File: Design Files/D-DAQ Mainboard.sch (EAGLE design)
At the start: 119 parts, among them Y1 XTC7009, Y2 DS1099

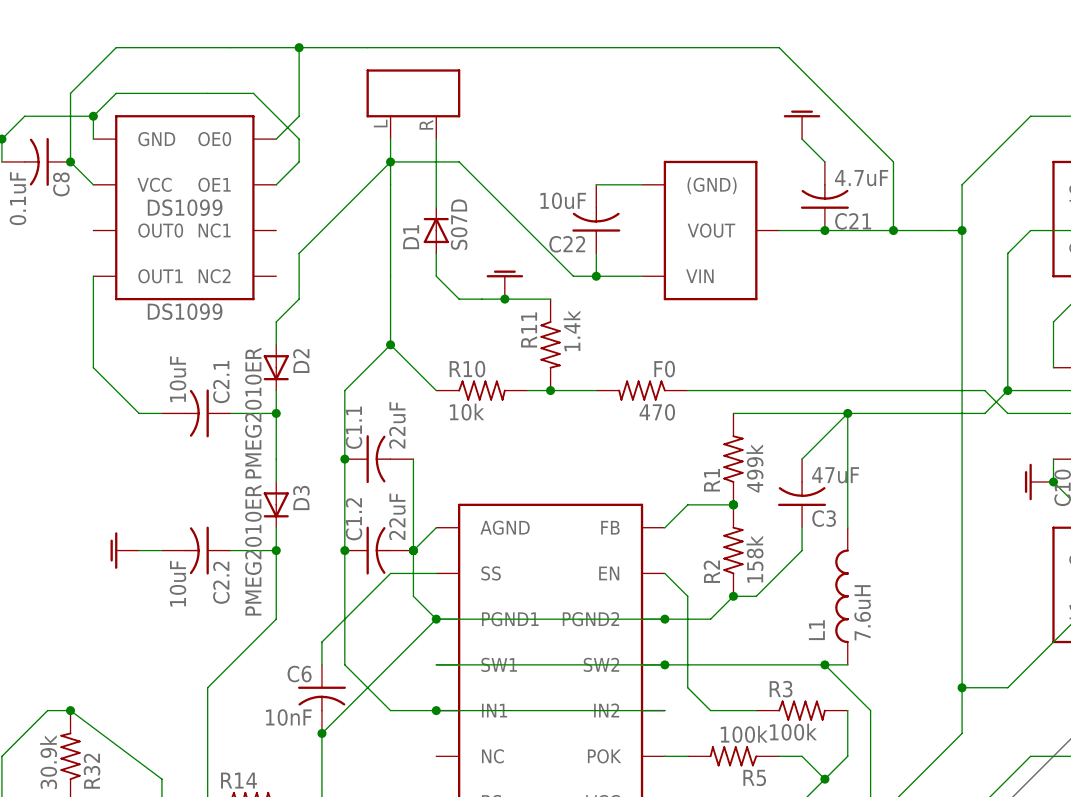
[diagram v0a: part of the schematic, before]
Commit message: v3.6.5 - Package & placement tweaks to design files and then permissions changes due to new system local copies reside
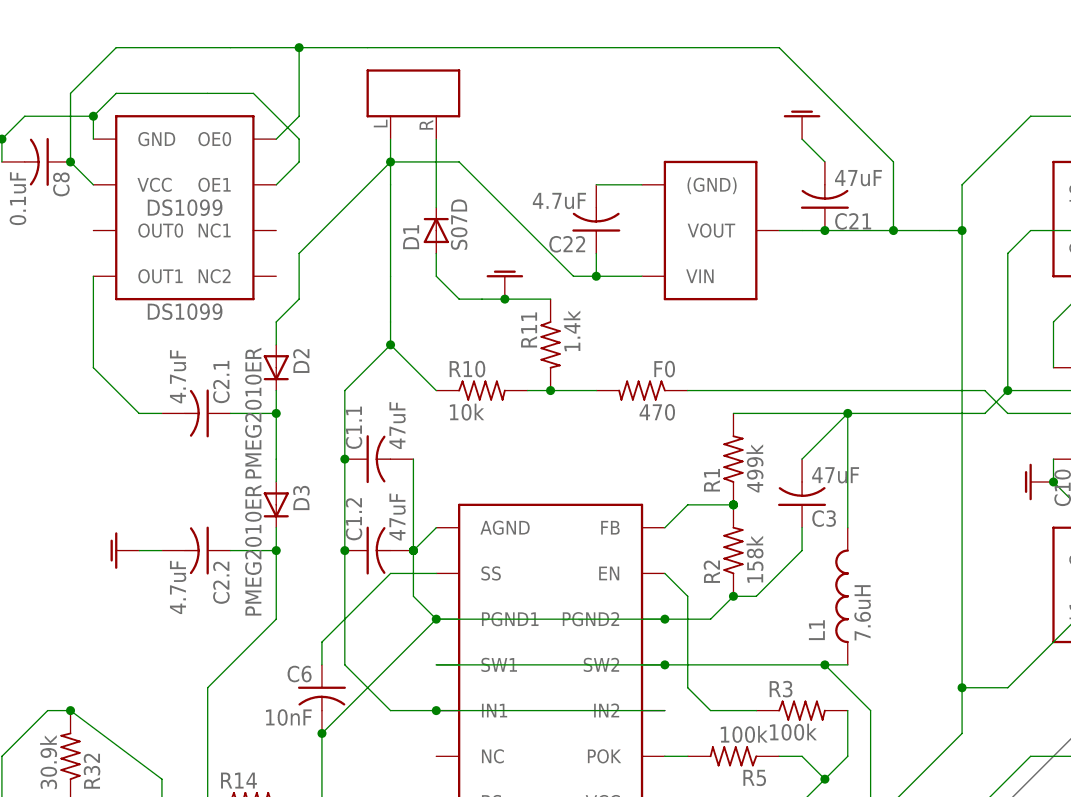
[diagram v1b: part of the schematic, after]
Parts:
- C1.1, C1.2: value 22uF -> 47uF
- C2.1, C2.2, C22: value 10uF -> 4.7uF; device Parts for D-DAQ:C-1210 -> Parts for D-DAQ:C-1206
- C21: value 4.7uF -> 47uF
- C31: device Parts for D-DAQ:C-1210 -> Parts for D-DAQ:C-1206
- renumbered 3.3V-TOGGLE-3 to 3.3V-TOGGLE-5, 5V-TOGGLE-3 to 5V-TOGGLE-5
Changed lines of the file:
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@@
 <part name="R131" library="Parts for D-DAQ" deviceset="R-" device="0603" value="255"/>
 <part name="R130" library="Parts for D-DAQ" deviceset="R-" device="0603" value="10k"/>
-<part name="C21" library="Parts for D-DAQ" deviceset="C-" device="1206" value="4.7uF"/>
-<part name="C22" library="Parts for D-DAQ" deviceset="C-" device="1210" value="10uF"/>
+<part name="C21" library="Parts for D-DAQ" deviceset="C-" device="1206" value="47uF"/>
+<part name="C22" library="Parts for D-DAQ" deviceset="C-" device="1206" value="4.7uF"/>
 <part name="GND-PIC2" library="supply1" deviceset="GNDA" device="" value=""/>
 <part name="R2" library="Parts for D-DAQ" deviceset="R-" device="0603" value="158k"/>
@@
 <part name="C5" library="Parts for D-DAQ" deviceset="C-" device="0603" value="0.1uF"/>
 <part name="C6" library="Parts for D-DAQ" deviceset="C-" device="0603" value="10nF"/>
-<part name="C1.1" library="Parts for D-DAQ" deviceset="C-" device="1812" value="22uF"/>
+<part name="C1.1" library="Parts for D-DAQ" deviceset="C-" device="1812" value="47uF"/>
 <part name="GND-PIC4" library="supply1" deviceset="GNDA" device="" value=""/>
 <part name="C3" library="Parts for D-DAQ" deviceset="C-" device="1206" value="47uF"/>
-<part name="C1.2" library="Parts for D-DAQ" deviceset="C-" device="1812" value="22uF"/>
+<part name="C1.2" library="Parts for D-DAQ" deviceset="C-" device="1812" value="47uF"/>
 <part name="C4" library="Parts for D-DAQ" deviceset="C-" device="0603" value="1uF"/>
 <part name="R31" library="Parts for D-DAQ" deviceset="R-" device="0603" value="3.01k"/>
 <part name="R32" library="Parts for D-DAQ" deviceset="R-" device="0603" value="30.9k"/>
-<part name="C31" library="Parts for D-DAQ" deviceset="C-" device="1210" value="10uF"/>
+<part name="C31" library="Parts for D-DAQ" deviceset="C-" device="1206" value="10uF"/>
 <part name="R4" library="Parts for D-DAQ" deviceset="R-" device="0603" value="10"/>
 <part name="R129" library="Parts for D-DAQ" deviceset="R-" device="0603" value="10k"/>
@@
 <part name="R12" library="Parts for D-DAQ" deviceset="R-" device="0603" value="10k"/>
 <part name="C7" library="Parts for D-DAQ" deviceset="C-" device="0603" value="0.1uF"/>
-<part name="C2.1" library="Parts for D-DAQ" deviceset="C-" device="1210" value="10uF"/>
+<part name="C2.1" library="Parts for D-DAQ" deviceset="C-" device="1206" value="4.7uF"/>
 <part name="Y2" library="Parts for D-DAQ" deviceset="DS1099" device="" value="DS1099"/>
-<part name="C2.2" library="Parts for D-DAQ" deviceset="C-" device="1210" value="10uF"/>
+<part name="C2.2" library="Parts for D-DAQ" deviceset="C-" device="1206" value="4.7uF"/>
 <part name="14V-REG" library="Parts for D-DAQ" deviceset="TL1963A-33DCQ" device=""/>
 <part name="GND-PIC5" library="supply1" deviceset="GNDA" device="" value=""/>
@@
 <part name="R20" library="Parts for D-DAQ" deviceset="R-" device="0603" value="100"/>
 <part name="JTAG" library="Parts for D-DAQ" deviceset="HEADER-X?" device="4"/>
-<part name="5V-TOGGLE-3" library="Parts for D-DAQ" deviceset="CPC1?17N" device="1" value="NC SSR"/>
-<part name="3.3V-TOGGLE-3" library="Parts for D-DAQ" deviceset="CPC1?17N" device="0" value="NO SSR"/>
+<part name="5V-TOGGLE-5" library="Parts for D-DAQ" deviceset="CPC1?17N" device="1" value="NC SSR"/>
+<part name="3.3V-TOGGLE-5" library="Parts for D-DAQ" deviceset="CPC1?17N" device="0" value="NO SSR"/>
 <part name="R15" library="Parts for D-DAQ" deviceset="R-" device="0603" value="100"/>
 <part name="D1" library="Parts for D-DAQ" deviceset="S07D" device=""/>
@@
 <instance part="R20" gate="G$1" x="-91.44" y="96.52" rot="R180"/>
 <instance part="JTAG" gate="G$1" x="15.24" y="-114.3" rot="MR270"/>
-<instance part="5V-TOGGLE-3" gate="G$1" x="-177.8" y="-48.26" rot="R180"/>
-<instance part="3.3V-TOGGLE-3" gate="G$1" x="-177.8" y="-35.56" rot="R180"/>
+<instance part="5V-TOGGLE-5" gate="G$1" x="-177.8" y="-48.26" rot="R180"/>
+<instance part="3.3V-TOGGLE-5" gate="G$1" x="-177.8" y="-35.56" rot="R180"/>
 <instance part="R15" gate="G$1" x="-58.42" y="17.78" rot="R180"/>
 <instance part="D1" gate="G$1" x="-165.1" y="111.76" rot="R90"/>
@@
 <wire x1="-203.2" y1="-17.78" x2="-203.2" y2="-40.64" width="0.1524" layer="91"/>
 <junction x="-195.58" y="-10.16"/>
-<pinref part="5V-TOGGLE-3" gate="G$1" pin="L2"/>
+<pinref part="5V-TOGGLE-5" gate="G$1" pin="L2"/>
 <wire x1="-203.2" y1="-40.64" x2="-193.04" y2="-50.8" width="0.1524" layer="91"/>
 <wire x1="-193.04" y1="-50.8" x2="-185.42" y2="-50.8" width="0.1524" layer="91"/>
@@
 <wire x1="-40.64" y1="88.9" x2="-40.64" y2="86.36" width="0.1524" layer="91"/>
 <wire x1="-40.64" y1="86.36" x2="-38.1" y2="83.82" width="0.1524" layer="91"/>
-<pinref part="3.3V-TOGGLE-3" gate="G$1" pin="L2"/>
+<pinref part="3.3V-TOGGLE-5" gate="G$1" pin="L2"/>
 <wire x1="-185.42" y1="-38.1" x2="-205.74" y2="-17.78" width="0.1524" layer="91"/>
 <wire x1="-205.74" y1="-17.78" x2="-205.74" y2="-15.24" width="0.1524" layer="91"/>
@@
 <wire x1="-162.56" y1="-12.7" x2="-162.56" y2="-30.48" width="0.1524" layer="91"/>
 <label x="-162.56" y="-30.48" size="1.778" layer="95" xref="yes"/>
-<pinref part="3.3V-TOGGLE-3" gate="G$1" pin="C-"/>
+<pinref part="3.3V-TOGGLE-5" gate="G$1" pin="C-"/>
 <wire x1="-167.64" y1="-33.02" x2="-165.1" y2="-30.48" width="0.1524" layer="91"/>
 <wire x1="-165.1" y1="-30.48" x2="-162.56" y2="-30.48" width="0.1524" layer="91"/>
@@
 <wire x1="-177.8" y1="-27.94" x2="-182.88" y2="-27.94" width="0.1524" layer="91"/>
 <wire x1="-182.88" y1="-27.94" x2="-185.42" y2="-30.48" width="0.1524" layer="91"/>
-<pinref part="3.3V-TOGGLE-3" gate="G$1" pin="L1"/>
+<pinref part="3.3V-TOGGLE-5" gate="G$1" pin="L1"/>
 <wire x1="-185.42" y1="-30.48" x2="-185.42" y2="-33.02" width="0.1524" layer="91"/>
-<pinref part="5V-TOGGLE-3" gate="G$1" pin="L1"/>
+<pinref part="5V-TOGGLE-5" gate="G$1" pin="L1"/>
 <wire x1="-185.42" y1="-45.72" x2="-187.96" y2="-43.18" width="0.1524" layer="91"/>
 <wire x1="-187.96" y1="-43.18" x2="-187.96" y2="-40.64" width="0.1524" layer="91"/>
@@
 </segment>
 <segment>
-<pinref part="5V-TOGGLE-3" gate="G$1" pin="C+"/>
+<pinref part="5V-TOGGLE-5" gate="G$1" pin="C+"/>
 <wire x1="-167.64" y1="-50.8" x2="-165.1" y2="-53.34" width="0.1524" layer="91"/>
 <label x="-165.1" y="-53.34" size="1.778" layer="95" xref="yes"/>
@@
 <net name="ICSP-SSR" class="0">
 <segment>
-<pinref part="5V-TOGGLE-3" gate="G$1" pin="C-"/>
-<pinref part="3.3V-TOGGLE-3" gate="G$1" pin="C+"/>
+<pinref part="5V-TOGGLE-5" gate="G$1" pin="C-"/>
+<pinref part="3.3V-TOGGLE-5" gate="G$1" pin="C+"/>
 <wire x1="-167.64" y1="-45.72" x2="-167.64" y2="-43.18" width="0.1524" layer="91"/>
 <wire x1="-167.64" y1="-43.18" x2="-167.64" y2="-40.64" width="0.1524" layer="91"/>
